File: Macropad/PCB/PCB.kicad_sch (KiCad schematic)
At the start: 26 parts, among them J1 USB_C_Receptacle_USB2.0_14P, J2 OLED_128x64, SW1 SW_Push, SW2 RotaryEncoder, SW3 RotaryEncoder, U1 STM32F072CBTx, U2 USBLC6-2SC6, U3 XC6206, U5 TRRS

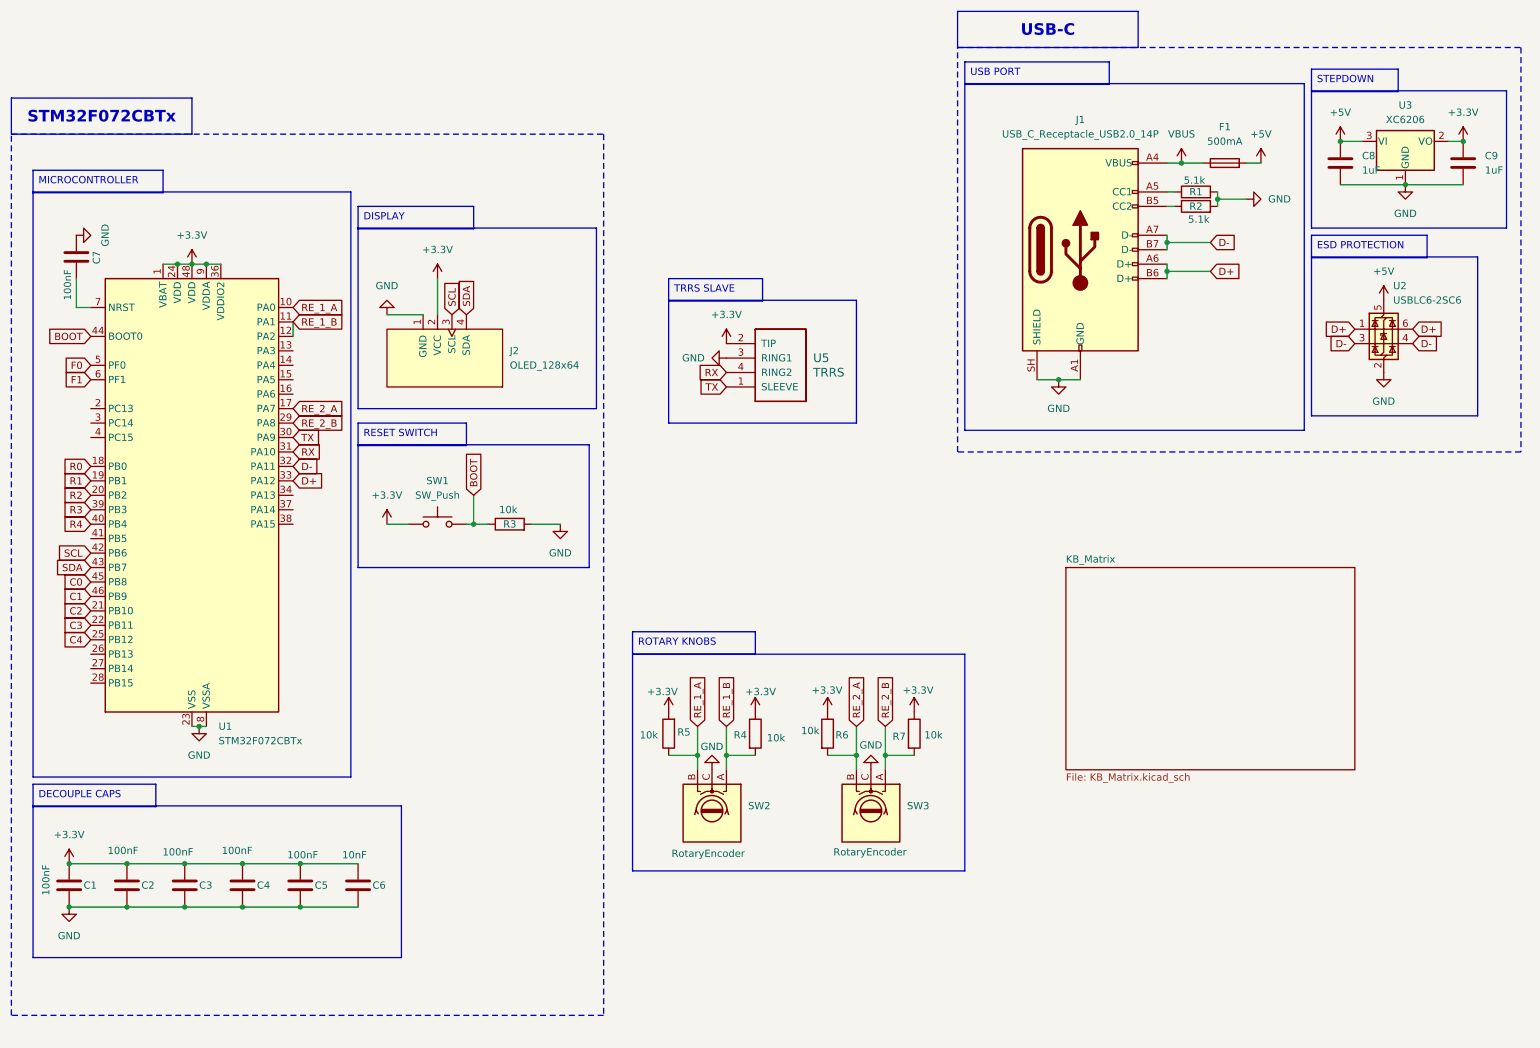
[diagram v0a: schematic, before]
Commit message: Updated code
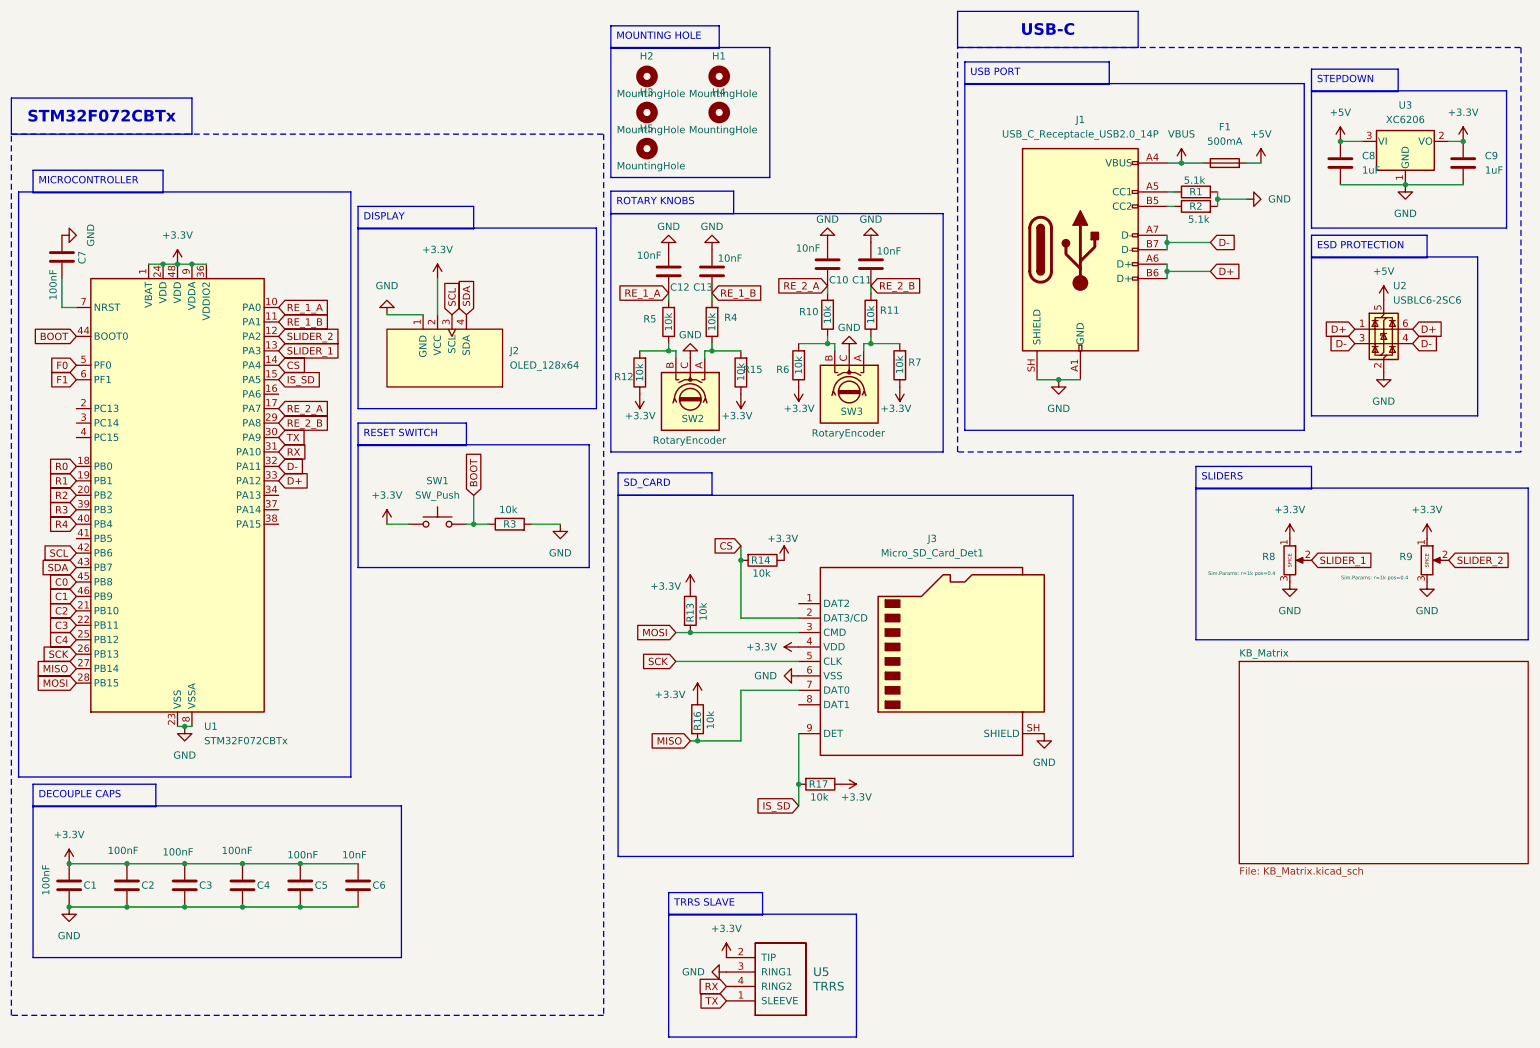
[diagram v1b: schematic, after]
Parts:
- added C10, C11, C12, C13: 10nF, Capacitor_SMD:C_0805_2012Metric, symbol Device:C
- added H1, H2, H3, H4, H5: MountingHole, MountingHole:MountingHole_2.7mm, symbol Mechanical:MountingHole
- added J3: Micro_SD_Card_Det1, symbol Connector:Micro_SD_Card_Det1
- added R10, R11, R12, R15: 10k, Resistor_SMD:R_0805_2012Metric, symbol ScottoKeebs:Placeholder_Resistor
- added R13, R14, R16, R17: 10k, symbol Device:R
- added R8, R9: Potentiometer, Potentiometer_THT:Potentiometer_Bourns_PTA6043_Single_Slide, symbol Simulation_SPICE:Potentiometer
- SW2, SW3: footprint Rotary_Encoder:RotaryEncoder_Alps_EC11E_Vertical_H20mm -> Rotary_Encoder:RotaryEncoder_Alps_EC12E-Switch_Vertical_H20mm
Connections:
- net +3.3V: now also J3.4 (VDD), R12.1, R13.1, R14.1, R15.1, R16.1, R17.1, R8.1, R9.1; no longer R4.1, R5.2
- net GND: now also C10.1, C11.1, C12.1, C13.1, J3.6 (VSS), J3.SH (SHIELD), R8.3, R9.3
- net RE_1_A: now also R5.2, C12.2; no longer R5.1, SW2.B
- net RE_1_B: now also C13.2; no longer SW2.A, U1.12 (PA2)
- net RE_2_A: now also C10.2, R10.2; no longer R6.2, SW3.B
- net RE_2_B: now also C11.2, R11.2; no longer R7.2, SW3.A
- net SLIDER_1: now reaches U1.13 (PA3)
- net SLIDER_1: now also R8.2
- net CS: now reaches U1.14 (PA4)
- net CS: now also J3.2 (DAT3/CD), R14.2
- net IS_SD: now reaches U1.15 (PA5)
- net IS_SD: now also J3.9 (DET), R17.2
- net SCK: now reaches U1.26 (PB13)
- net SCK: now also J3.5 (CLK)
- net MISO: now reaches U1.27 (PB14)
- net MISO: now also J3.7 (DAT0), R16.2
- net MOSI: now reaches U1.28 (PB15)
- net MOSI: now also J3.3 (CMD), R13.2
- new net: R11.1, R7.2, SW3.A
- new net: R10.1, R6.2, SW3.B
- new net: R15.2, R4.1, SW2.A
- new net: R12.2, R5.1, SW2.B
- new net SLIDER_2: R9.2, U1.12 (PA2)
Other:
- moved on the sheet: C7, U1, U5
